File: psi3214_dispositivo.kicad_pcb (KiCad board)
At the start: 2 copper layers, 51.5 x 67 mm, 25 parts, among them J2 AudioJack3, J4 Conn_01x03, J5 AudioJack3, U1 TL072_sim, U2 MAX1044

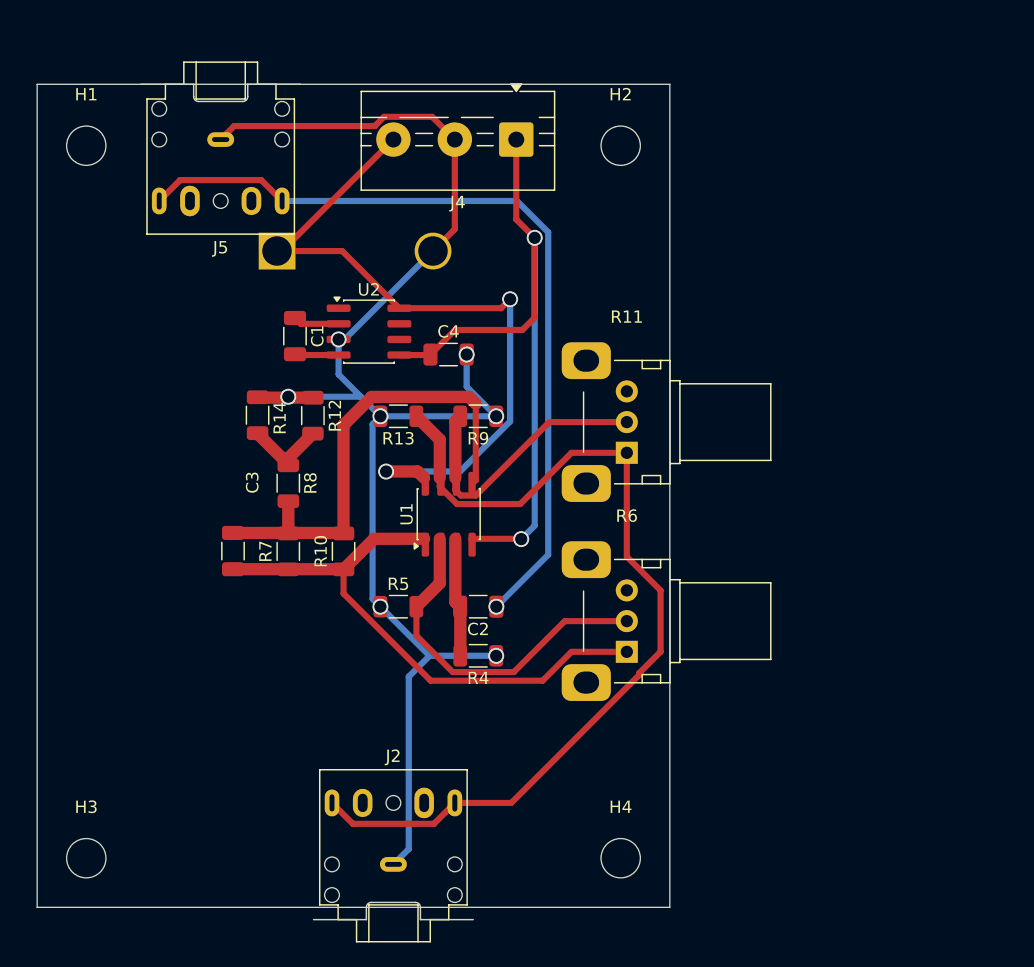
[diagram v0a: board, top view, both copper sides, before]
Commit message: kinda broken state
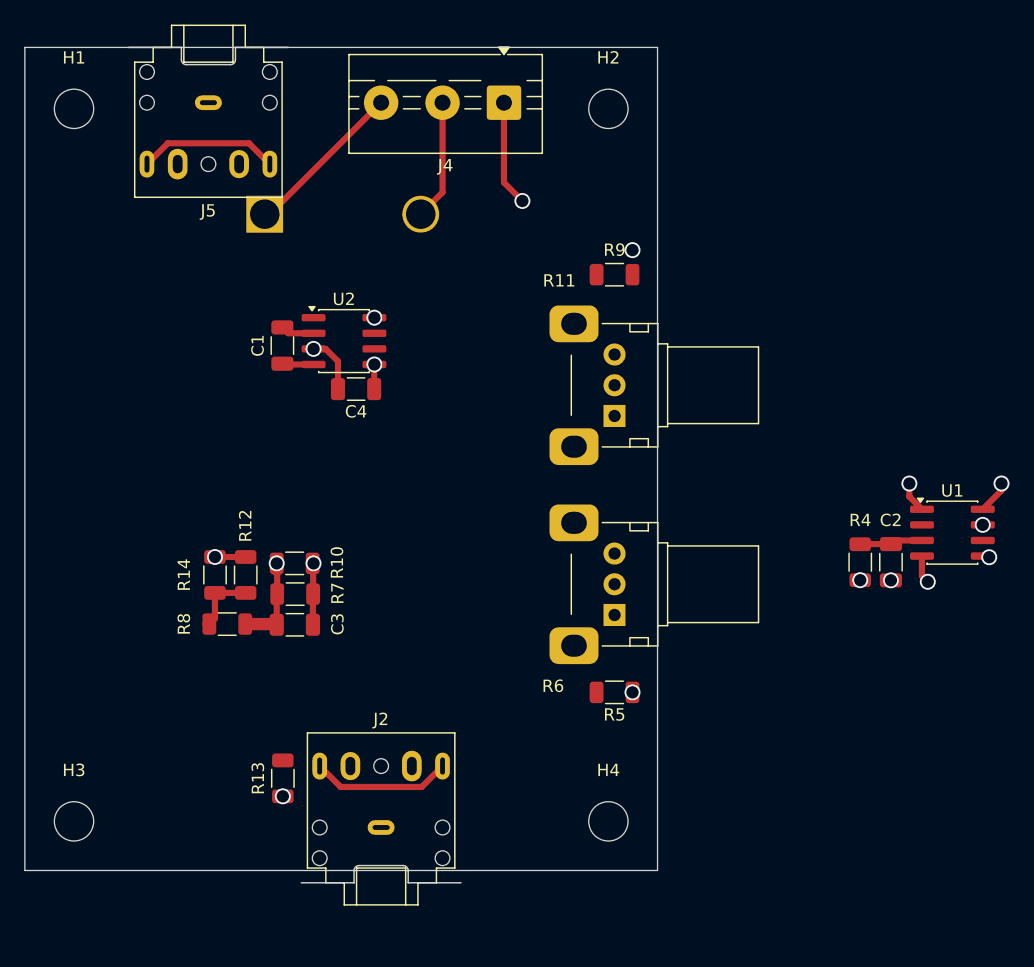
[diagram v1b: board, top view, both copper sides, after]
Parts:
- moved U1 41.0 mm to (200.5, 107.0), turned to 0 degrees
- moved C2 33.8 mm to (195.5, 109.4), turned to 90 degrees
- moved R4 32.0 mm to (193.0, 109.4), turned to 90 degrees
- moved R13 30.9 mm to (146.0, 127.0), turned to -90 degrees
- moved R5 18.9 mm to (173.0, 120.0), turned to 180 degrees
- moved R9 16.0 mm to (173.0, 86.0)
- moved R12 14.1 mm to (143.0, 110.4)
- moved R14 13.5 mm to (140.5, 110.4)
- moved R8 12.5 mm to (141.5, 114.4), turned to 0 degrees
- moved C4 8.03 mm to (152.0, 95.3), turned to 180 degrees
- moved C3 7.83 mm to (147.0, 114.5), turned to 180 degrees
- moved R10 4.10 mm to (147.0, 109.5), turned to 180 degrees
- moved R7 3.52 mm to (147.0, 112.0), turned to 180 degrees
- moved BT1 3.16 mm to (144.5, 81.1)
- moved H1 3.16 mm to (129.0, 72.5)
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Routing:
- net GND: track 120.3 -> 17.5 mm, vias 7 -> 6
- net saida: track 74.7 -> 11.4 mm, vias 0 -> 1
- net entrada: track 66.4 -> 11.4 mm
- net -9V: track 56.4 -> 12.9 mm, vias 2 -> 3
- net +9V: track 59.4 -> 16.0 mm
- net saida_amp1: track 45.5 -> 7.54 mm, vias 0 -> 2
- net saida_filtro: track 39.8 -> 8.22 mm, vias 0 -> 2
- net Net-(U1A--): track 28.8 -> 0.00 mm
- net Net-(U1B--): track 22.8 -> 0.00 mm
- net saida_cap: track 9.69 -> 5.76 mm
- net Net-(R12-Pad2): track 7.01 -> 5.30 mm
- net Net-(U2-CAP-): track 3.58 -> 2.56 mm
- net Net-(U2-CAP+): track 3.75 -> 2.73 mm
